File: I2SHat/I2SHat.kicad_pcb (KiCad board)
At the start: 4 copper layers, 65 x 56 mm, 98 parts, among them J1 TORX142L, J2 TOTX142L, J3 TX_RCA, J4 Raspberry_Pi_2_3, J5 RX_RCA, Q1 BSS138, Q2 BSS138, Q3 BSS138, Q4 BSS138, Q5 BSS138, SW1 GW12RCP, U1 74LVC1G125DBV, U10 LD1117S33, U11 LD1117S33, U2 NC7SZ157P6X, U3 74LVC1G125DBV, U4 74LVC1G125DBV, U5 74LVC1GU04DBV, U6 74LV1T04DBV, U7 WM8804, U8 SN74LV1T34DBV, U9 LD1117S33, Y1 ABMM-12.000MHZ

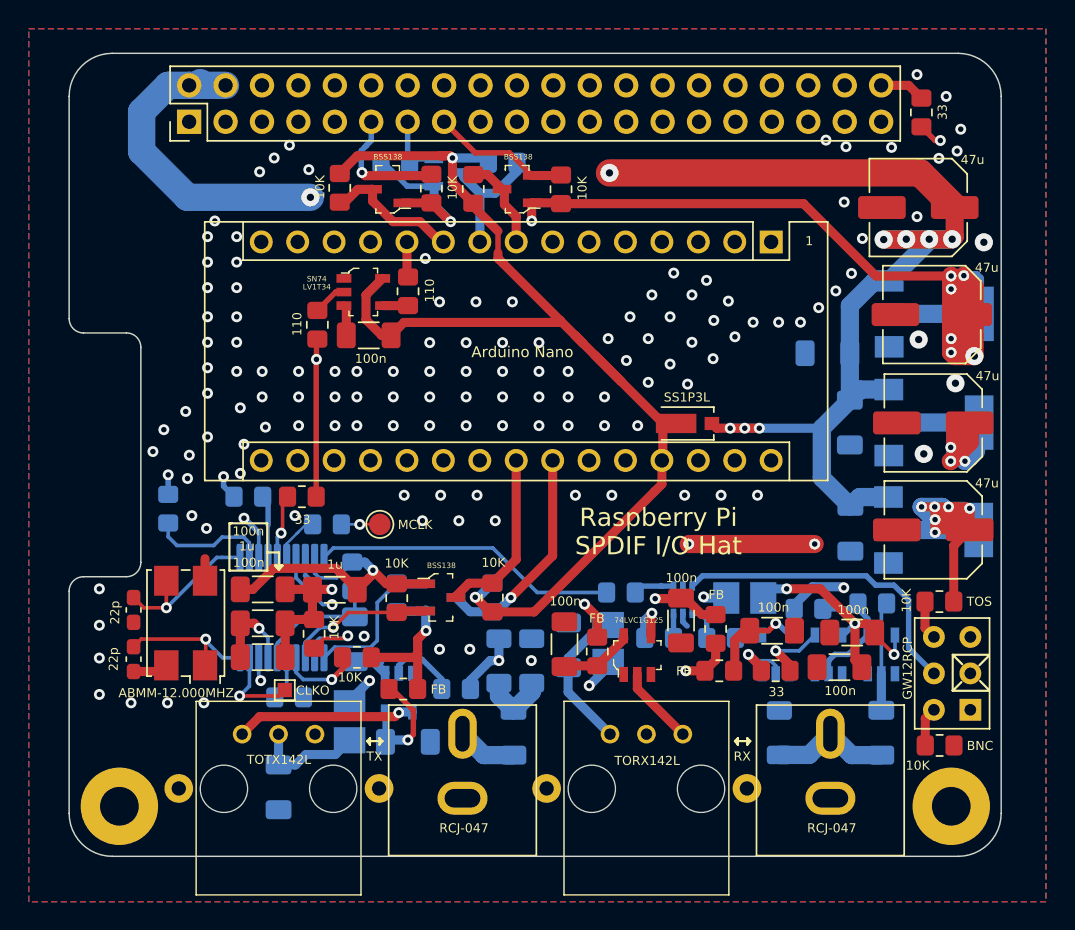
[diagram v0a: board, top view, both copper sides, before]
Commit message: WIP changes
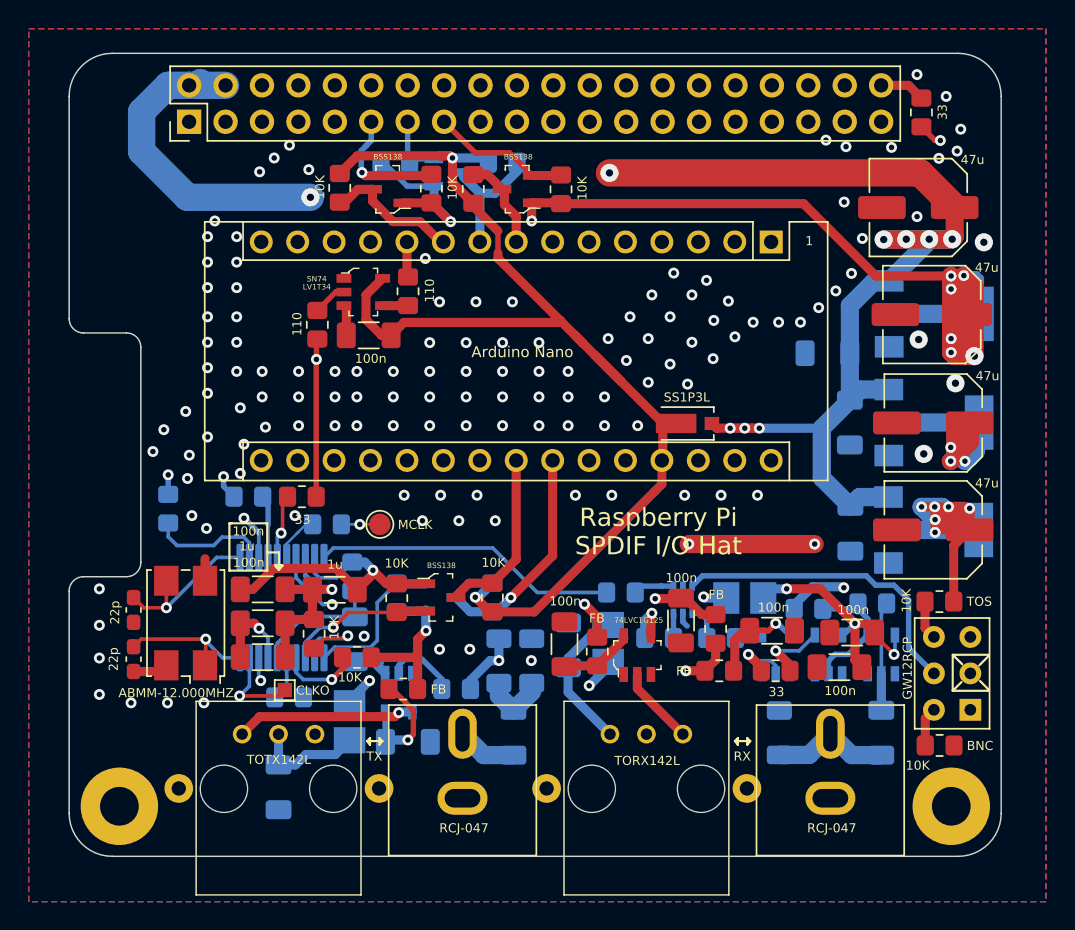
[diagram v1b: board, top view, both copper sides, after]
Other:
- net class Default removed
